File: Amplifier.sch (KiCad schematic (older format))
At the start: 58 parts, among them J501 TB001-500-04BE CUI_Devices, Q401 2N7002, Q402 2N7002, SW501 DS04-254-2-02BK-SMT, U501 TDA7498L

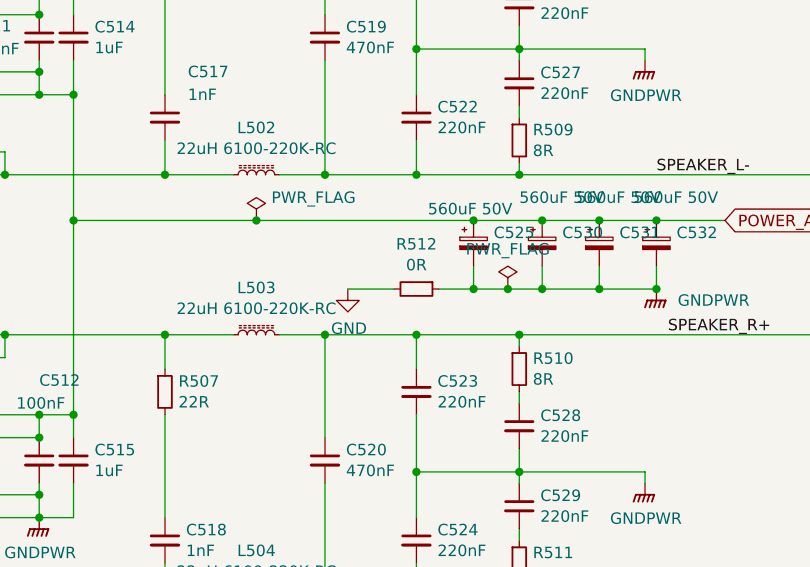
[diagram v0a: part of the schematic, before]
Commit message: Nach Änderungen auf der Arbeit + anderes
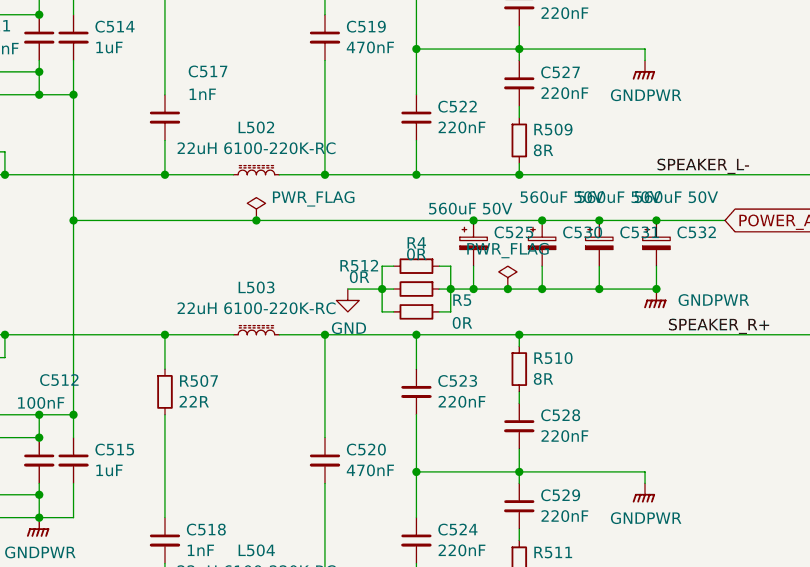
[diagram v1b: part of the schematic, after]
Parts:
- added R4, R5: 0R, Resistor_SMD:R_1206_3216Metric_Pad1.42x1.75mm_HandSolder, symbol Device:R_Small
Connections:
- net GND: now also R4.2, R5.2
- net GNDPWR: now also R4.1, R5.1
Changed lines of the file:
@@
 U 1 1 5EC064F0
 P 8000 3800
-F 0 "R512" V 7804 3800 50  0000 C CNN
-F 1 "0R" V 7895 3800 50  0000 C CNN
+F 0 "R512" V 7900 3550 50  0000 C CNN
+F 1 "0R" V 7950 3550 50  0000 C CNN
 F 2 "Resistor_SMD:R_1206_3216Metric_Pad1.42x1.75mm_HandSolder" H 8000 3800 50  0001 C CNN
 F 3 "~" H 8000 3800 50  0001 C CNN
@@
 $EndComp
 Wire Wire Line
-	8100 3800 8250 3800
+	8100 3800 8150 3800
 $Comp
 L power:PWR_FLAG #FLG0111
@@
 $EndComp
 Wire Wire Line
-	7700 3800 7900 3800
+	7700 3800 7850 3800
 $Comp
 L Device:CP_Small C525
@@
 Connection ~ 2750 6450
 Connection ~ 3550 7050
+$Comp
+L Device:R_Small R5
+U 1 1 5ED99689
+P 8000 3900
+F 0 "R5" V 7950 4100 50  0000 C CNN
+F 1 "0R" V 8050 4100 50  0000 C CNN
+F 2 "Resistor_SMD:R_1206_3216Metric_Pad1.42x1.75mm_HandSolder" H 8000 3900 50  0001 C CNN
+F 3 "~" H 8000 3900 50  0001 C CNN
+	1    8000 3900
+	0    1    1    0
+$EndComp
+$Comp
+L Device:R_Small R4
+U 1 1 5ED99910
+P 8000 3700
+F 0 "R4" V 7900 3700 50  0000 C CNN
+F 1 "0R" V 7950 3700 50  0000 C CNN
+F 2 "Resistor_SMD:R_1206_3216Metric_Pad1.42x1.75mm_HandSolder" H 8000 3700 50  0001 C CNN
+F 3 "~" H 8000 3700 50  0001 C CNN
+	1    8000 3700
+	0    1    1    0
+$EndComp
+Wire Wire Line
+	8100 3700 8150 3700
+Wire Wire Line
+	8150 3700 8150 3800
+Connection ~ 8150 3800
+Wire Wire Line
+	8150 3800 8250 3800
+Wire Wire Line
+	8100 3900 8150 3900
+Wire Wire Line
+	8150 3900 8150 3800
+Wire Wire Line
+	7900 3700 7850 3700
+Wire Wire Line
+	7850 3700 7850 3800
+Connection ~ 7850 3800
+Wire Wire Line
+	7850 3800 7900 3800
+Wire Wire Line
+	7900 3900 7850 3900
+Wire Wire Line
+	7850 3900 7850 3800
 $EndSCHEMATC
